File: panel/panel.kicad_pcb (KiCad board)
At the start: 4 copper layers, 36 x 36 mm, 288 parts, among them J1 IN, J2 OUT, Q1 Q_PMOS_GSD, Q10 Q_PMOS_GSD, Q11 Q_PMOS_GSD, Q12 Q_PMOS_GSD, Q13 Q_PMOS_GSD, Q14 Q_PMOS_GSD, Q15 Q_PMOS_GSD, Q16 Q_PMOS_GSD, Q2 Q_PMOS_GSD, Q3 Q_PMOS_GSD, Q4 Q_PMOS_GSD, Q5 Q_PMOS_GSD, Q6 Q_PMOS_GSD, Q7 Q_PMOS_GSD, Q8 Q_PMOS_GSD, Q9 Q_PMOS_GSD, U1 TLC59025, U2 TLC59025, U3 TLC59025, U4 SN74HC595, U5 SN74HC595, U6 NC7WZ17, U7 NC7WZ17

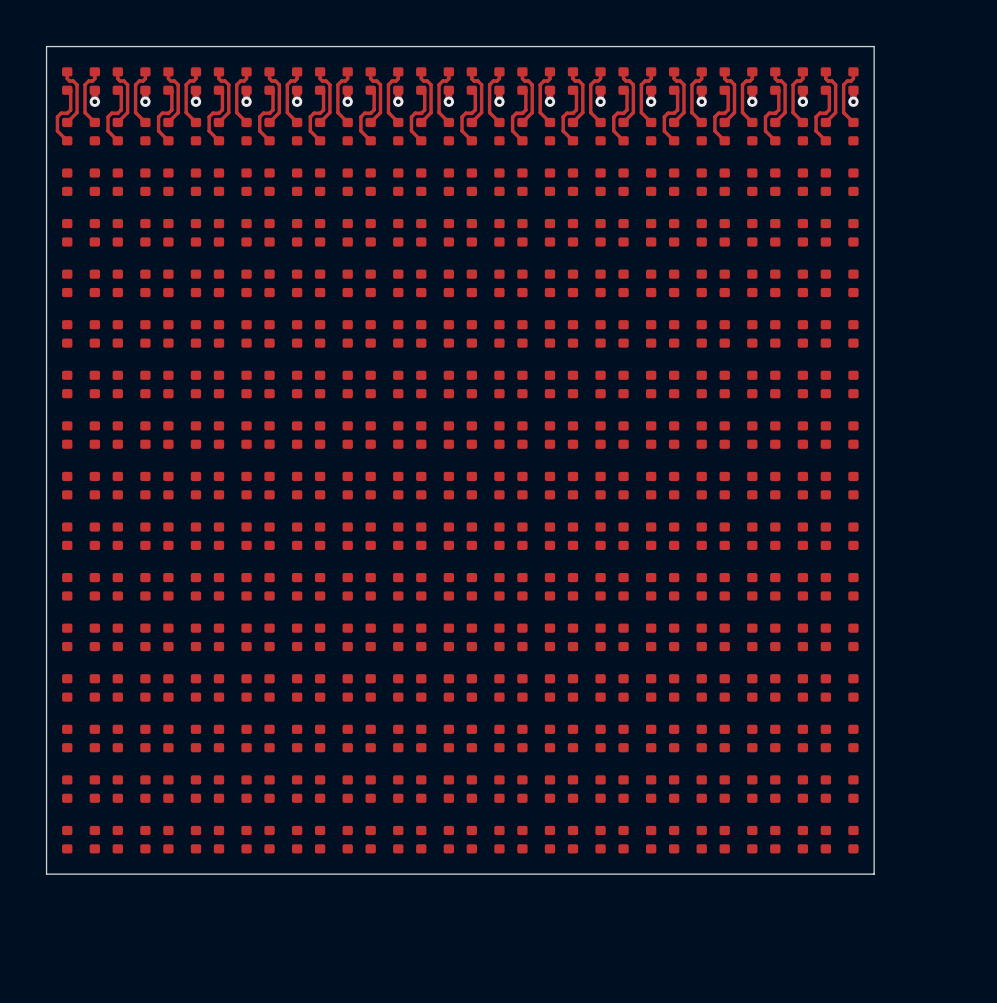
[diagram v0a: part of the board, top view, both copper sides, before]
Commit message: Routed columns
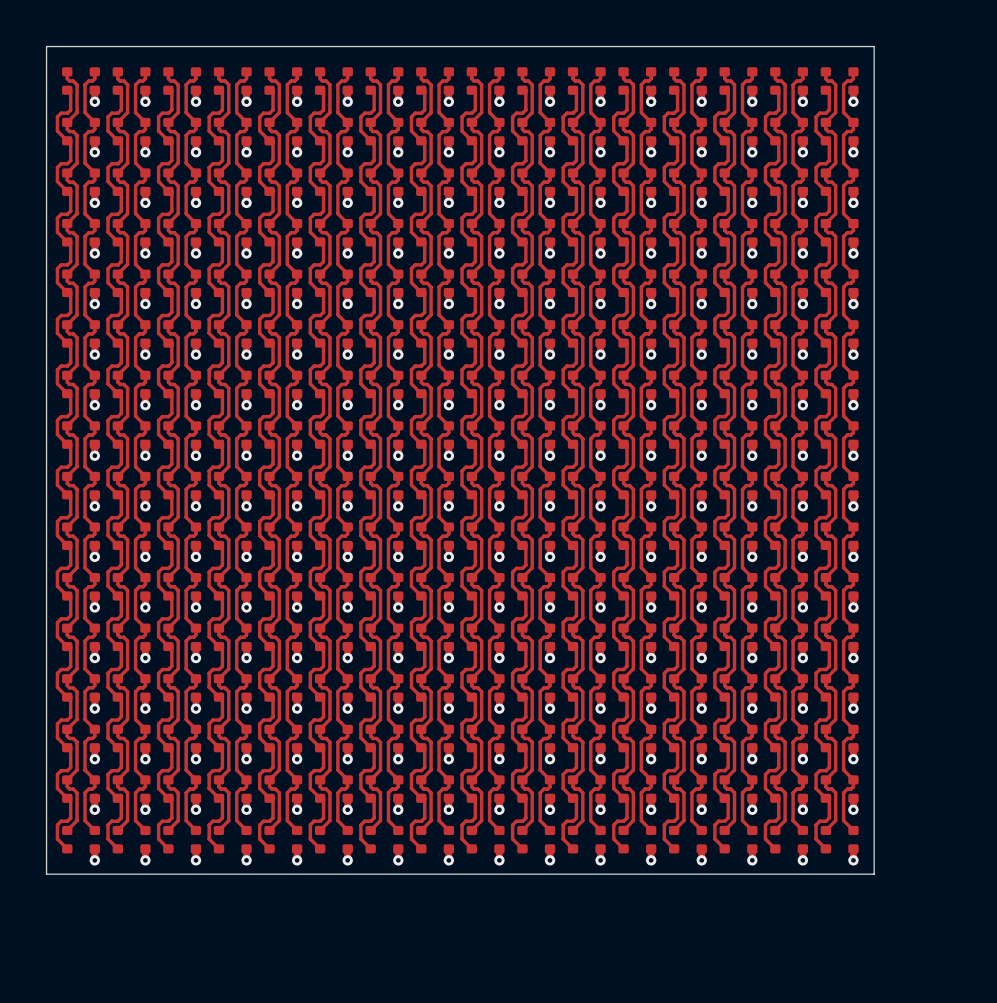
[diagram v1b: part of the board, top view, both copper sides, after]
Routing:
- net COL_9B: track 2.92 -> 44.0 mm
- net COL_15B: track 2.92 -> 44.0 mm
- net COL_5B: track 2.92 -> 44.0 mm
- net COL_14B: track 2.92 -> 44.0 mm
- net COL_10B: track 2.92 -> 44.0 mm
- net COL_4B: track 2.92 -> 44.0 mm
- net COL_1B: track 2.92 -> 44.0 mm
- net COL_2B: track 2.92 -> 44.0 mm
- net COL_8B: track 2.92 -> 44.0 mm
- net COL_7B: track 2.92 -> 44.0 mm
- net COL_3B: track 2.92 -> 44.0 mm
- net COL_13B: track 2.92 -> 44.0 mm
- net COL_12B: track 2.92 -> 44.0 mm
- net COL_0B: track 2.92 -> 44.0 mm
- net COL_6B: track 2.92 -> 44.0 mm
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
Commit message: Routed rows
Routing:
- net /ROW_2/COMMON: track 8.00 -> 49.4 mm
- net /ROW_13/COMMON: track 8.00 -> 49.4 mm
- net /ROW_8/COMMON: track 8.00 -> 49.4 mm
- net /ROW_7/COMMON: track 8.00 -> 49.4 mm
- net /ROW_1/COMMON: track 8.00 -> 49.4 mm
- net /ROW_6/COMMON: track 8.00 -> 49.4 mm
- net /ROW_3/COMMON: track 8.00 -> 49.4 mm
- net /ROW_12/COMMON: track 8.00 -> 49.4 mm
- net /ROW_11/COMMON: track 8.00 -> 49.4 mm
- net /ROW_0/COMMON: track 8.00 -> 49.4 mm
- net /ROW_9/COMMON: track 8.00 -> 49.4 mm
- net /ROW_4/COMMON: track 8.00 -> 49.4 mm
- net /ROW_14/COMMON: track 8.00 -> 49.4 mm
- net /ROW_5/COMMON: track 8.00 -> 49.4 mm
- net /ROW_10/COMMON: track 8.00 -> 49.4 mm
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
